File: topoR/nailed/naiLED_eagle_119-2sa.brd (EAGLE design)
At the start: 12.4 x 14 mm, 9 parts, among them IC1 TCS3414

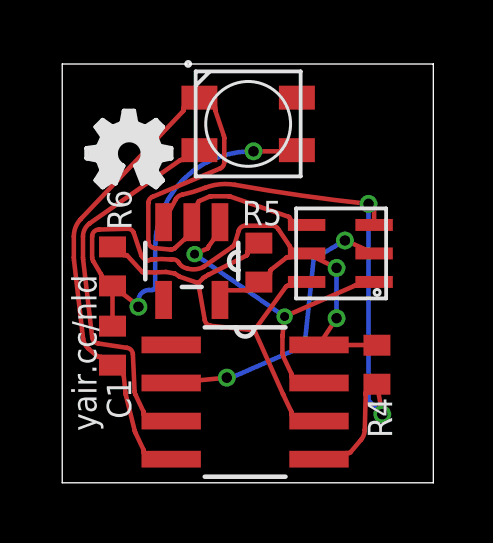
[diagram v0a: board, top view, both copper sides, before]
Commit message: sent to fab, single board
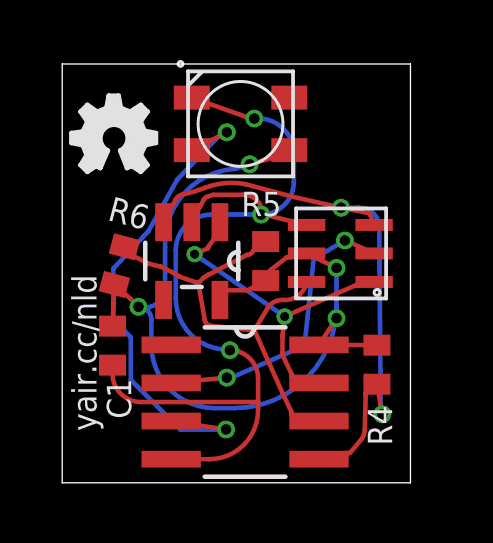
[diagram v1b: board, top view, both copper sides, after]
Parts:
- moved E$1 0.72 mm to (0.30, 10.4)
- moved U$1 0.25 mm to (5.94, 12.0)
- moved R5 0.23 mm to (6.78, 7.39)
- moved R6 0.23 mm to (1.91, 7.24), turned to 75 degrees
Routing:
- net D4/PWM: track 12.9 -> 17.3 mm, vias 0 -> 2
- net GND: track 29.2 -> 30.5 mm, vias 0 -> 3
- net VCC: track 31.1 -> 30.0 mm
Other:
- board size 12.4 x 14 mm -> 11.6 x 14 mm
